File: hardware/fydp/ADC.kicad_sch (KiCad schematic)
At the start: 31 parts, among them J20 Conn_01x07_Pin, U34 LTC2353ILX-16-PBF

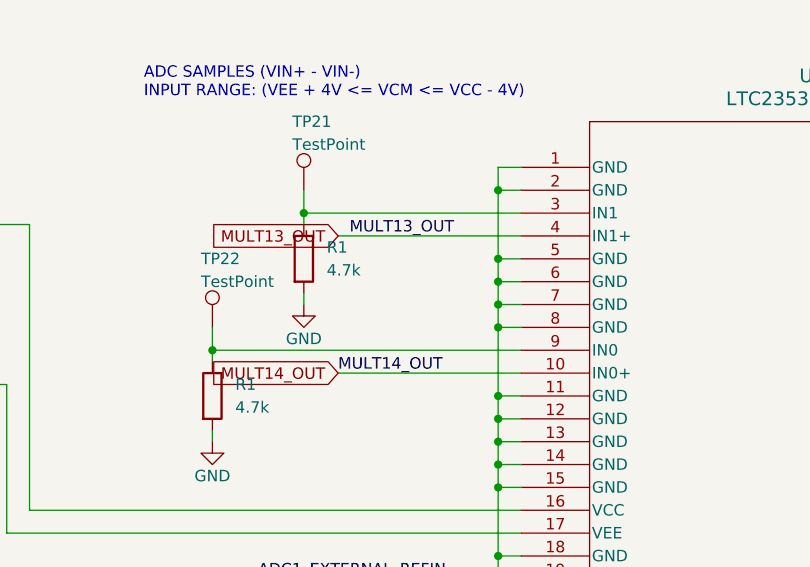
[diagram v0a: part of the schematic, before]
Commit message: Pushing all changes, I'm late for class
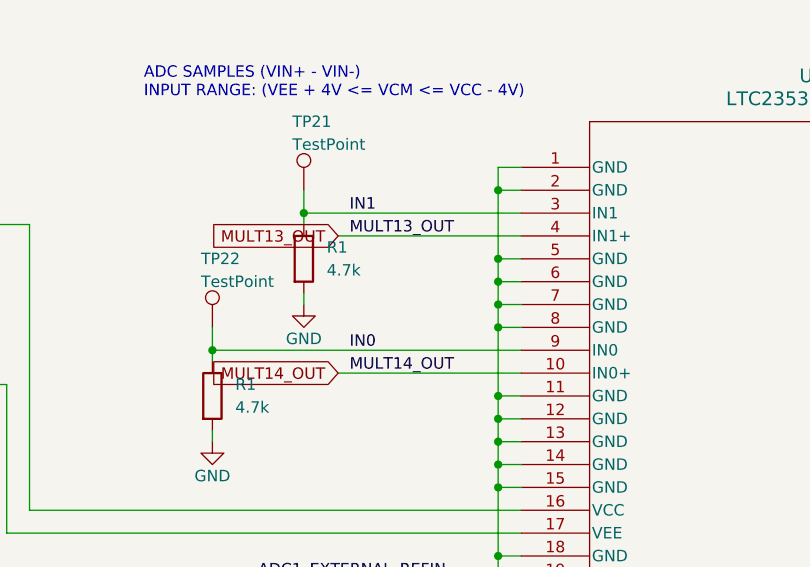
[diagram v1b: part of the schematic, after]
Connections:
- net IN0: now reaches R1.1, TP22.1, U34.9 (IN0)
- net IN1: now reaches R1.1, TP21.1, U34.3 (IN1)
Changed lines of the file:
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@@
     (effects (font (size 1.27 1.27)) (justify left bottom))
   )
-  (label "MULT14_OUT" (at 96.52 67.31 0) (fields_autoplaced)
+  (label "MULT14_OUT" (at 97.79 67.31 0) (fields_autoplaced)
     (effects (font (size 1.27 1.27)) (justify left bottom))
   )
@@
     (effects (font (size 1.27 1.27)) (justify left bottom))
   )
+  (label "IN1" (at 97.79 49.53 0) (fields_autoplaced)
+    (effects (font (size 1.27 1.27)) (justify left bottom))
+  )
   (label "ADC1_VDDLBYP" (at 233.68 41.91 0) (fields_autoplaced)
     (effects (font (size 1.27 1.27)) (justify left bottom))
@@
     (effects (font (size 1.27 1.27)) (justify left bottom))
   )
+  (label "IN0" (at 97.79 64.77 0) (fields_autoplaced)
+    (effects (font (size 1.27 1.27)) (justify left bottom))
+  )
